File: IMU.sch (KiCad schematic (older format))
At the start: 6 parts, among them U12 MPU-9250

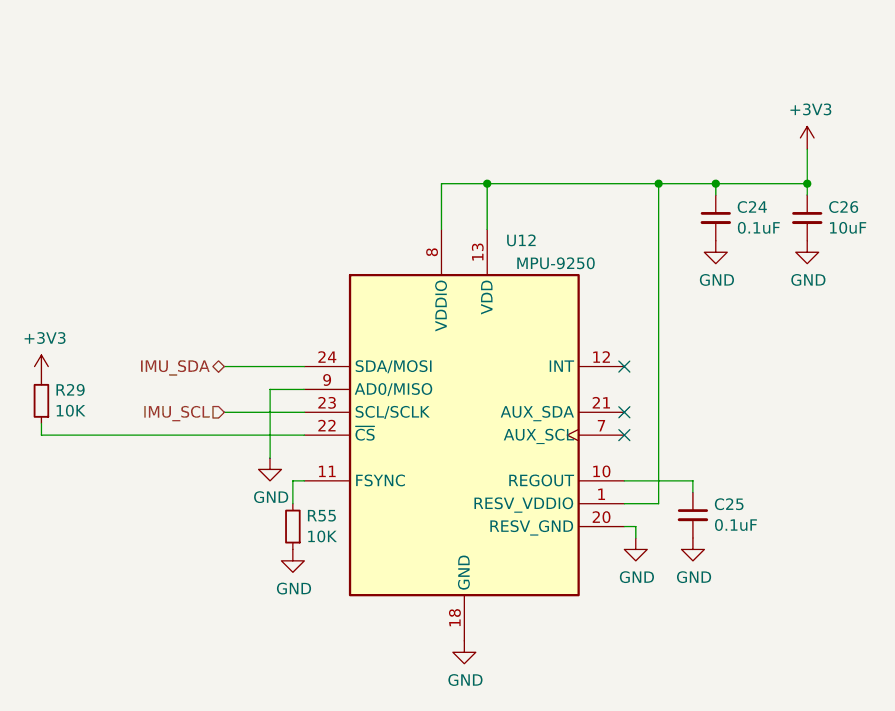
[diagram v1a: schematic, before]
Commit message: NXP version
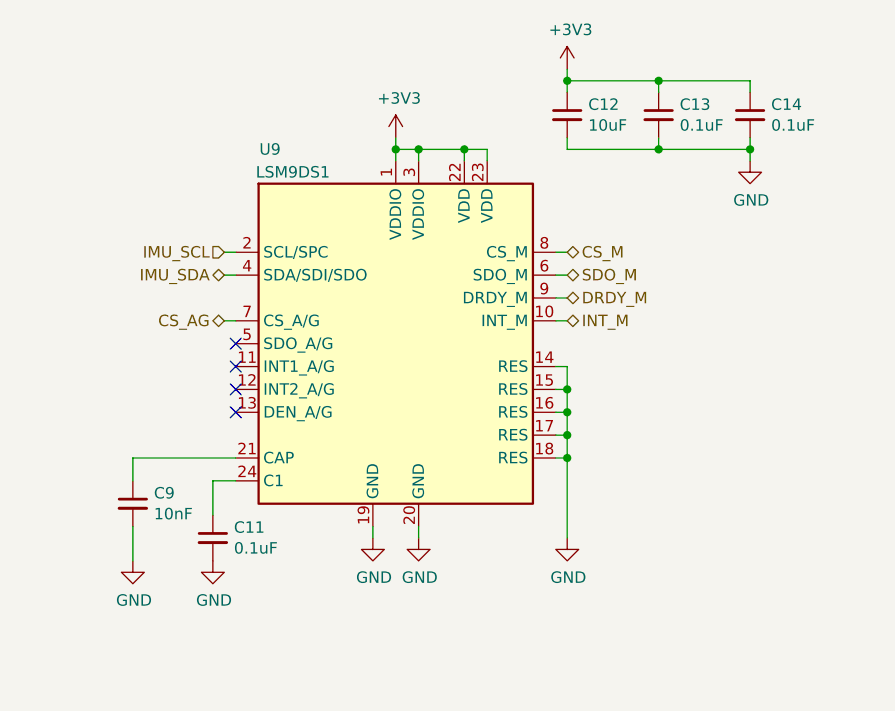
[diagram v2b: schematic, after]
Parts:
- removed C24, C25: 0.1uF, Capacitor_SMD:C_0402_1005Metric, symbol Device:C_Small
- removed C26: 10uF, Capacitor_SMD:C_0603_1608Metric, symbol Device:C_Small
- removed R29, R55: 10K, Resistor_SMD:R_0402_1005Metric, symbol Device:R_Small
- removed U12: MPU-9250, Sensor_Motion:InvenSense_QFN-24_3x3mm_P0.4mm, symbol Sensor_Motion:MPU-9250
- added C11, C13, C14: 0.1uF, Capacitor_SMD:C_0402_1005Metric, symbol Device:C_Small
- added C12: 10uF, Capacitor_SMD:C_0402_1005Metric, symbol Device:C_Small
- added C9: 10nF, Capacitor_SMD:C_0603_1608Metric, symbol Device:C_Small
- added U9: LSM9DS1, Package_LGA:LGA-24L_3x3.5mm_P0.43mm, symbol Sensor_Motion:LSM9DS1
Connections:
- net +3V3: now also C12.1, C13.1, C14.1, U9.1 (VDDIO), U9.22 (VDD), U9.23 (VDD), U9.3 (VDDIO)
- net GND: now also C11.2, C12.2, C13.2, C14.2, C9.2, U9.14 (RES), U9.15 (RES), U9.16 (RES), U9.17 (RES), U9.18 (RES), U9.19 (GND), U9.20 (GND)
- net IMU_SCL: now also U9.2 (SCL/SPC)
- net IMU_SDA: now also U9.4 (SDA/SDI/SDO)
- new net: C9.1, U9.21 (CAP)
- new net: C11.1, U9.24 (C1)
- new net CS_AG: U9.7 (CS_A/G)
- new net CS_M: U9.8 (CS_M)
- new net DRDY_M: U9.9 (DRDY_M)
- new net INT_M: U9.10 (INT_M)
- new net SDO_M: U9.6 (SDO_M)
- no-connect marks 3 -> 4
